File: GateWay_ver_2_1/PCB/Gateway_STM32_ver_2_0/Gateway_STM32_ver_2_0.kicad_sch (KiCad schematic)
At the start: 44 parts, among them J4 Conn_01x04, SW2 SW_Push, U7 STM32F407VETx, Y1 8mhz, Y2 Crystal_GND23

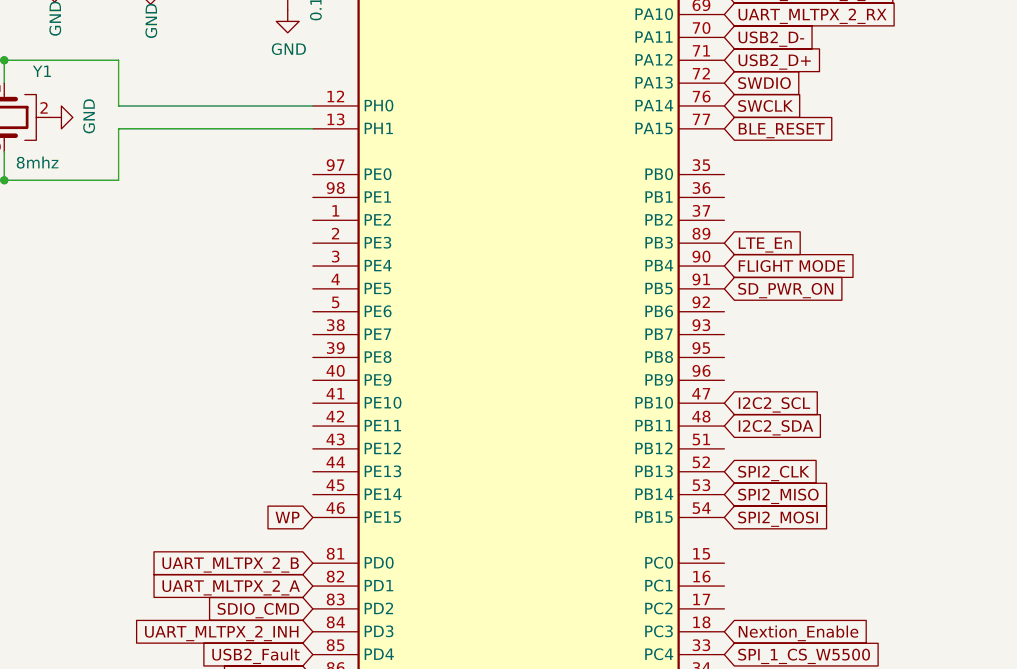
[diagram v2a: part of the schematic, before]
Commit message: 1
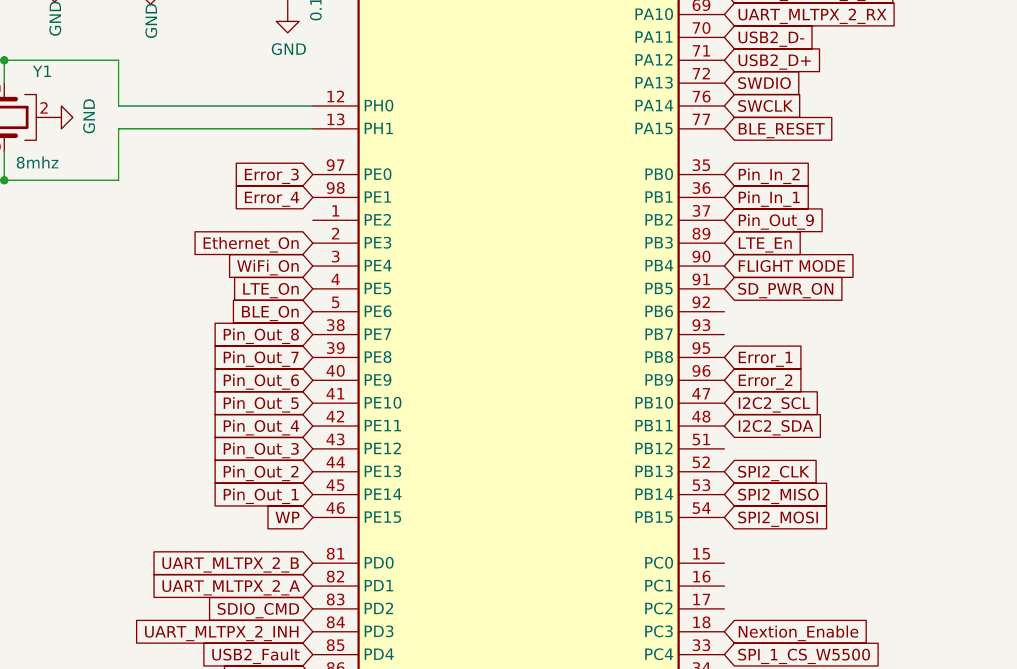
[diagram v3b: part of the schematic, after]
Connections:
- net BLE_On: now also U7.5 (PE6)
- net Error_1: now also U7.95 (PB8)
- net Error_2: now also U7.96 (PB9)
- net Error_3: now also U7.97 (PE0)
- net Error_4: now also U7.98 (PE1)
- net Ethernet_On: now also U7.2 (PE3)
- net LTE_On: now also U7.4 (PE5)
- net WiFi_On: now also U7.3 (PE4)
- net Pin_In_2: now reaches U7.35 (PB0)
- net Pin_In_1: now reaches U7.36 (PB1)
- net Pin_Out_9: now reaches U7.37 (PB2)
- net Pin_Out_8: now reaches U7.38 (PE7)
- net Pin_Out_7: now reaches U7.39 (PE8)
- net Pin_Out_6: now reaches U7.40 (PE9)
- net Pin_Out_5: now reaches U7.41 (PE10)
- net Pin_Out_4: now reaches U7.42 (PE11)
- net Pin_Out_3: now reaches U7.43 (PE12)
- net Pin_Out_2: now reaches U7.44 (PE13)
- net Pin_Out_1: now reaches U7.45 (PE14)
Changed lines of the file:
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@@
     (effects (font (size 5.0038 5.0038) (thickness 1.0008) bold) (justify left bottom))
   )
+  (global_label "Pin_Out_1" (shape input) (at 68.326 130.048 180) (fields_autoplaced)
+    (effects (font (size 1.27 1.27)) (justify right))
+    (property "Intersheet References" "${INTERSHEET_REFS}" (id 0) (at 56.628 130.1274 0)
+      (effects (font (size 1.27 1.27)) (justify right) hide)
+    )
+  )
   (global_label "SDIO_CK" (shape input) (at 114.046 168.148 0) (fields_autoplaced)
     (effects (font (size 1.27 1.27)) (justify left))
@@
     )
   )
+  (global_label "Pin_In_2" (shape input) (at 114.046 94.488 0) (fields_autoplaced)
+    (effects (font (size 1.27 1.27)) (justify left))
+    (property "Intersheet References" "${INTERSHEET_REFS}" (id 0) (at 124.2926 94.4086 0)
+      (effects (font (size 1.27 1.27)) (justify left) hide)
+    )
+  )
   (global_label "LTE_RXD" (shape input) (at 68.326 152.908 180) (fields_autoplaced)
     (effects (font (size 1.27 1.27)) (justify right))
@@
     )
   )
+  (global_label "Pin_Out_2" (shape input) (at 68.326 127.508 180) (fields_autoplaced)
+    (effects (font (size 1.27 1.27)) (justify right))
+    (property "Intersheet References" "${INTERSHEET_REFS}" (id 0) (at 56.628 127.4286 0)
+      (effects (font (size 1.27 1.27)) (justify right) hide)
+    )
+  )
+  (global_label "Pin_Out_6" (shape input) (at 68.326 117.348 180) (fields_autoplaced)
+    (effects (font (size 1.27 1.27)) (justify right))
+    (property "Intersheet References" "${INTERSHEET_REFS}" (id 0) (at 56.628 117.2686 0)
+      (effects (font (size 1.27 1.27)) (justify right) hide)
+    )
+  )
+  (global_label "Pin_Out_8" (shape input) (at 68.326 112.268 180) (fields_autoplaced)
+    (effects (font (size 1.27 1.27)) (justify right))
+    (property "Intersheet References" "${INTERSHEET_REFS}" (id 0) (at 56.628 112.1886 0)
+      (effects (font (size 1.27 1.27)) (justify right) hide)
+    )
+  )
   (global_label "Nextion_Rx" (shape input) (at 114.046 53.848 0) (fields_autoplaced)
     (effects (font (size 1.27 1.27)) (justify left))
@@
     )
   )
+  (global_label "Pin_In_1" (shape input) (at 114.046 97.028 0) (fields_autoplaced)
+    (effects (font (size 1.27 1.27)) (justify left))
+    (property "Intersheet References" "${INTERSHEET_REFS}" (id 0) (at 124.2926 97.1074 0)
+      (effects (font (size 1.27 1.27)) (justify left) hide)
+    )
+  )
   (global_label "Error_2" (shape input) (at 228.473 48.26 180) (fields_autoplaced)
     (effects (font (size 1.27 1.27)) (justify right))
@@
     )
   )
+  (global_label "Error_2" (shape input) (at 114.046 117.348 0) (fields_autoplaced)
+    (effects (font (size 1.27 1.27)) (justify left))
+    (property "Intersheet References" "${INTERSHEET_REFS}" (id 0) (at 475.361 665.353 0)
+      (effects (font (size 1.27 1.27)) hide)
+    )
+  )
   (global_label "LTE_En" (shape input) (at 114.046 102.108 0) (fields_autoplaced)
     (effects (font (size 1.27 1.27)) (justify left))
@@
     )
   )
+  (global_label "LTE_On" (shape input) (at 68.326 107.188 180) (fields_autoplaced)
+    (effects (font (size 1.27 1.27)) (justify right))
+    (property "Intersheet References" "${INTERSHEET_REFS}" (id 0) (at -246.634 -448.437 0)
+      (effects (font (size 1.27 1.27)) hide)
+    )
+  )
   (global_label "FLIGHT MODE" (shape input) (at 114.046 104.648 0) (fields_autoplaced)
     (effects (font (size 1.27 1.27)) (justify left))
@@
     )
   )
+  (global_label "Error_3" (shape input) (at 68.326 94.488 180) (fields_autoplaced)
+    (effects (font (size 1.27 1.27)) (justify right))
+    (property "Intersheet References" "${INTERSHEET_REFS}" (id 0) (at -292.989 -460.502 0)
+      (effects (font (size 1.27 1.27)) hide)
+    )
+  )
   (global_label "UART_MLTPX_1_INH" (shape input) (at 68.326 170.688 180) (fields_autoplaced)
     (effects (font (size 1.27 1.27)) (justify right))
@@
     )
   )
+  (global_label "Ethernet_On" (shape input) (at 68.326 102.108 180) (fields_autoplaced)
+    (effects (font (size 1.27 1.27)) (justify right))
+    (property "Intersheet References" "${INTERSHEET_REFS}" (id 0) (at -246.634 -439.547 0)
+      (effects (font (size 1.27 1.27)) hide)
+    )
+  )
   (global_label "Error_1" (shape input) (at 228.473 41.275 180) (fields_autoplaced)
     (effects (font (size 1.27 1.27)) (justify right))
@@
     )
   )
+  (global_label "BLE_On" (shape input) (at 68.326 109.728 180) (fields_autoplaced)
+    (effects (font (size 1.27 1.27)) (justify right))
+    (property "Intersheet References" "${INTERSHEET_REFS}" (id 0) (at -246.634 -452.882 0)
+      (effects (font (size 1.27 1.27)) hide)
+    )
+  )
+  (global_label "Pin_Out_3" (shape input) (at 68.326 124.968 180) (fields_autoplaced)
+    (effects (font (size 1.27 1.27)) (justify right))
+    (property "Intersheet References" "${INTERSHEET_REFS}" (id 0) (at 56.628 125.0474 0)
+      (effects (font (size 1.27 1.27)) (justify right) hide)
+    )
+  )
   (global_label "Nextion_Enable" (shape input) (at 114.046 145.288 0) (fields_autoplaced)
     (effects (font (size 1.27 1.27)) (justify left))
@@
     )
   )
+  (global_label "Error_1" (shape input) (at 114.046 114.808 0) (fields_autoplaced)
+    (effects (font (size 1.27 1.27)) (justify left))
+    (property "Intersheet References" "${INTERSHEET_REFS}" (id 0) (at 475.361 655.828 0)
+      (effects (font (size 1.27 1.27)) hide)
+    )
+  )
   (global_label "UART_MLTPX_2_A" (shape input) (at 68.326 140.208 180) (fields_autoplaced)
     (effects (font (size 1.27 1.27)) (justify right))
@@
     )
   )
+  (global_label "Pin_Out_4" (shape input) (at 68.326 122.428 180) (fields_autoplaced)
+    (effects (font (size 1.27 1.27)) (justify right))
+    (property "Intersheet References" "${INTERSHEET_REFS}" (id 0) (at 56.628 122.3486 0)
+      (effects (font (size 1.27 1.27)) (justify right) hide)
+    )
+  )
   (global_label "SPI2_CLK" (shape input) (at 114.046 127.508 0) (fields_autoplaced)
     (effects (font (size 1.27 1.27)) (justify left))
@@
     )
   )
+  (global_label "Pin_Out_5" (shape input) (at 68.326 119.888 180) (fields_autoplaced)
+    (effects (font (size 1.27 1.27)) (justify right))
+    (property "Intersheet References" "${INTERSHEET_REFS}" (id 0) (at 56.628 119.9674 0)
+      (effects (font (size 1.27 1.27)) (justify right) hide)
+    )
+  )
   (global_label "SDIO_D1" (shape input) (at 114.046 160.528 0) (fields_autoplaced)
     (effects (font (size 1.27 1.27)) (justify left))
@@
     )
   )
+  (global_label "WiFi_On" (shape input) (at 68.326 104.648 180) (fields_autoplaced)
+    (effects (font (size 1.27 1.27)) (justify right))
+    (property "Intersheet References" "${INTERSHEET_REFS}" (id 0) (at -246.634 -443.992 0)
+      (effects (font (size 1.27 1.27)) hide)
+    )
+  )
   (global_label "Nextion_Tx" (shape input) (at 114.046 51.308 0) (fields_autoplaced)
     (effects (font (size 1.27 1.27)) (justify left))
@@
     )
   )
+  (global_label "Pin_Out_9" (shape input) (at 114.046 99.568 0) (fields_autoplaced)
+    (effects (font (size 1.27 1.27)) (justify left))
+    (property "Intersheet References" "${INTERSHEET_REFS}" (id 0) (at 125.744 99.4886 0)
+      (effects (font (size 1.27 1.27)) (justify left) hide)
+    )
+  )
   (global_label "SWCLK" (shape input) (at 114.046 86.868 0) (fields_autoplaced)
     (effects (font (size 1.27 1.27)) (justify left))
@@
     )
   )
+  (global_label "Error_4" (shape input) (at 68.326 97.028 180) (fields_autoplaced)
+    (effects (font (size 1.27 1.27)) (justify right))
+    (property "Intersheet References" "${INTERSHEET_REFS}" (id 0) (at -292.989 -464.947 0)
+      (effects (font (size 1.27 1.27)) hide)
+    )
+  )
   (global_label "UART_MLTPX_1_TX" (shape input) (at 68.326 157.988 180) (fields_autoplaced)
     (effects (font (size 1.27 1.27)) (justify right))
@@
     )
   )
+  (global_label "Pin_Out_7" (shape input) (at 68.326 114.808 180) (fields_autoplaced)
+    (effects (font (size 1.27 1.27)) (justify right))
+    (property "Intersheet References" "${INTERSHEET_REFS}" (id 0) (at 56.628 114.8874 0)
+      (effects (font (size 1.27 1.27)) (justify right) hide)
+    )
+  )
